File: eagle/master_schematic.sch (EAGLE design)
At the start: 110 parts

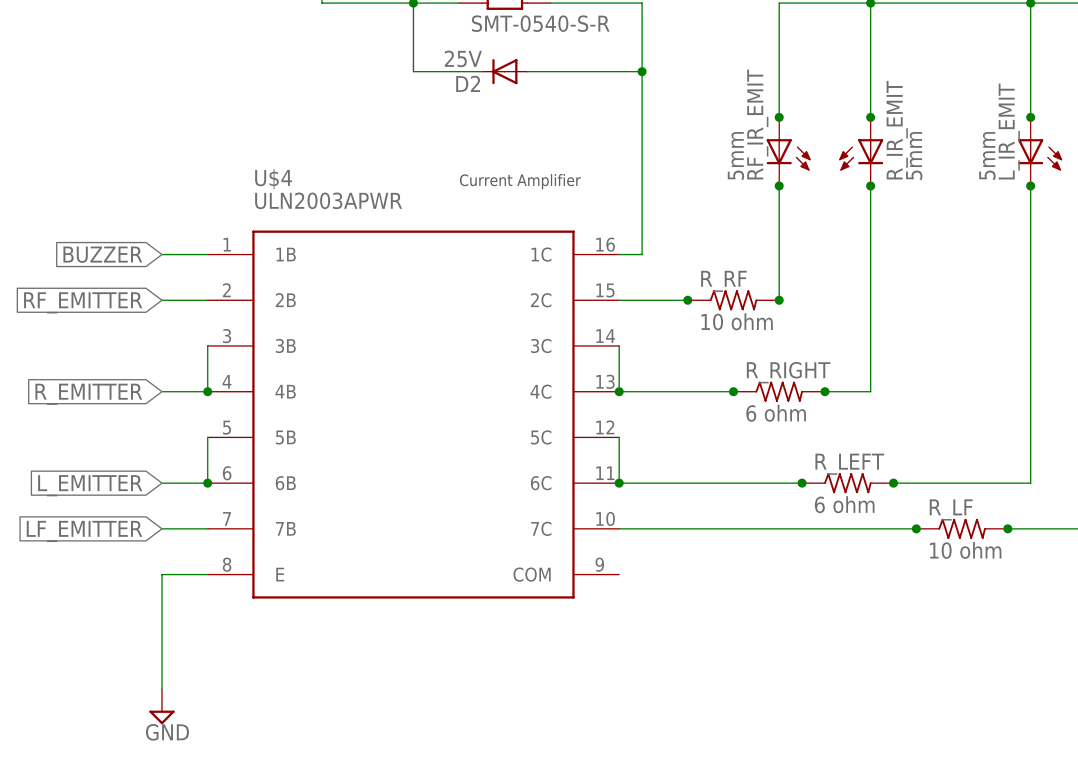
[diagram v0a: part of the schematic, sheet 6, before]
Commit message: ULN and stuff
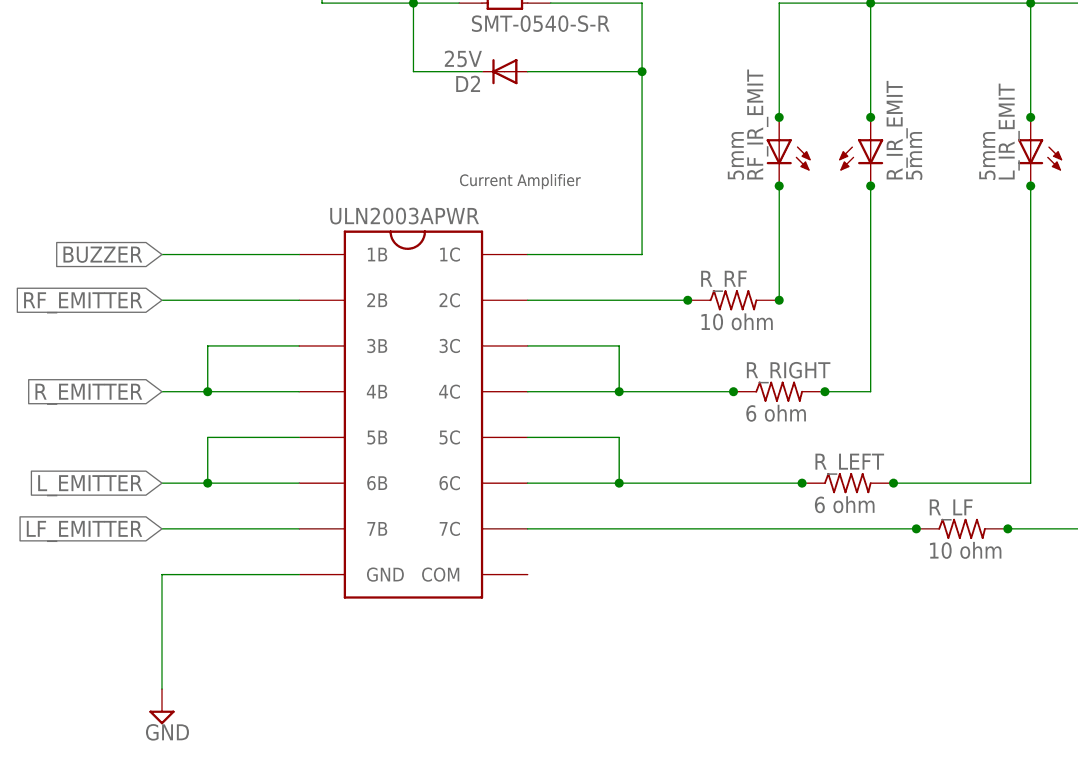
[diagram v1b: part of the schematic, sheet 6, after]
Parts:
- removed U$4: ULN2003APWR, MMULN:ULN2003APWR
- added U$9: ULN2003APWR, ULN2003APWR:ULN2003APWR
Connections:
- net BUZZER: now also U$9.1B; no longer U$4.1B
- net GND: now also U$9.GND; no longer U$4.E
- net LF_EMITTER: now also U$9.7B; no longer U$4.7B
- net L_EMITTER: now also U$9.5B, U$9.6B; no longer U$4.5B, U$4.6B
- net N$22: now also U$9.2C; no longer U$4.2C
- net N$24: now also U$9.3C, U$9.4C; no longer U$4.3C, U$4.4C
- net N$27: now also U$9.5C, U$9.6C; no longer U$4.5C, U$4.6C
- net N$29: now also U$9.1C; no longer U$4.1C
- net N$30: now also U$9.7C; no longer U$4.7C
- net RF_EMITTER: now also U$9.2B; no longer U$4.2B
- net R_EMITTER: now also U$9.3B, U$9.4B; no longer U$4.3B, U$4.4B
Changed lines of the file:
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@@
 <part name="C1_F_EMITS" library="resistor" deviceset="C-EU" device="C1206" value="4.7uF"/>
 <part name="C2_F_EMITS" library="resistor" deviceset="C-EU" device="C1206" value=".1uF"/>
-<part name="U$4" library="MMULN" deviceset="ULN2003APWR" device=""/>
 <part name="R_MOT" library="pinhead" deviceset="PINHD-2X3" device=""/>
 <part name="L_MOT" library="pinhead" deviceset="PINHD-2X3" device=""/>
@@
 <part name="U$7" library="JST_CONNECTOR_FEMALE. through hole" deviceset="JST_CONNECTOR_FEMALE" device=""/>
 <part name="U$8" library="JST_CONNECTOR_FEMALE. through hole" deviceset="JST_CONNECTOR_FEMALE" device=""/>
+<part name="U$9" library="ULN2003APWR" deviceset="ULN2003APWR" device=""/>
 </parts>
 <sheets>
@@
 <instance part="C1_F_EMITS" gate="G$1" x="147.32" y="27.94" rot="R180"/>
 <instance part="C2_F_EMITS" gate="G$1" x="165.1" y="27.94" rot="R180"/>
-<instance part="U$4" gate="G$1" x="-17.78" y="0"/>
 <instance part="SUPPLY10" gate="GND" x="81.28" y="-17.78"/>
 <instance part="SUPPLY11" gate="GND" x="-45.72" y="-33.02"/>
@@
 <instance part="SPK1" gate="G$1" x="-7.62" y="45.72"/>
 <instance part="D2" gate="G$1" x="-7.62" y="38.1" rot="R180"/>
+<instance part="U$9" gate="G$1" x="-17.78" y="-2.54"/>
 </instances>
 <busses>
@@
 <net name="RF_EMITTER" class="0">
 <segment>
-<wire x1="-45.72" y1="12.7" x2="-40.64" y2="12.7" width="0.1524" layer="91"/>
 <label x="-45.72" y="12.7" size="1.778" layer="95" rot="R180" xref="yes"/>
-<pinref part="U$4" gate="G$1" pin="2B"/>
+<pinref part="U$9" gate="G$1" pin="2B"/>
+<wire x1="-45.72" y1="12.7" x2="-30.48" y2="12.7" width="0.1524" layer="91"/>
 </segment>
 </net>
@@
 <wire x1="-40.64" y1="2.54" x2="-40.64" y2="7.62" width="0.1524" layer="91"/>
 <label x="-45.72" y="2.54" size="1.778" layer="95" rot="R180" xref="yes"/>
-<pinref part="U$4" gate="G$1" pin="3B"/>
-<pinref part="U$4" gate="G$1" pin="4B"/>
+<pinref part="U$9" gate="G$1" pin="3B"/>
+<wire x1="-40.64" y1="7.62" x2="-30.48" y2="7.62" width="0.1524" layer="91"/>
+<pinref part="U$9" gate="G$1" pin="4B"/>
+<wire x1="-40.64" y1="2.54" x2="-30.48" y2="2.54" width="0.1524" layer="91"/>
 <junction x="-40.64" y="2.54"/>
 </segment>
@@
 <wire x1="-40.64" y1="-7.62" x2="-40.64" y2="-2.54" width="0.1524" layer="91"/>
 <label x="-45.72" y="-7.62" size="1.778" layer="95" rot="R180" xref="yes"/>
-<pinref part="U$4" gate="G$1" pin="5B"/>
-<pinref part="U$4" gate="G$1" pin="6B"/>
+<pinref part="U$9" gate="G$1" pin="5B"/>
+<wire x1="-40.64" y1="-2.54" x2="-30.48" y2="-2.54" width="0.1524" layer="91"/>
+<pinref part="U$9" gate="G$1" pin="6B"/>
+<wire x1="-40.64" y1="-7.62" x2="-30.48" y2="-7.62" width="0.1524" layer="91"/>
 <junction x="-40.64" y="-7.62"/>
 </segment>
@@
 <net name="LF_EMITTER" class="0">
 <segment>
-<wire x1="-40.64" y1="-12.7" x2="-45.72" y2="-12.7" width="0.1524" layer="91"/>
 <label x="-45.72" y="-12.7" size="1.778" layer="95" rot="R180" xref="yes"/>
-<pinref part="U$4" gate="G$1" pin="7B"/>
+<pinref part="U$9" gate="G$1" pin="7B"/>
+<wire x1="-45.72" y1="-12.7" x2="-30.48" y2="-12.7" width="0.1524" layer="91"/>
 </segment>
 </net>
@@
 <pinref part="R_RF" gate="G$1" pin="1"/>
 <junction x="12.7" y="12.7"/>
-<wire x1="12.7" y1="12.7" x2="5.08" y2="12.7" width="0.1524" layer="91"/>
-<pinref part="U$4" gate="G$1" pin="2C"/>
+<pinref part="U$9" gate="G$1" pin="2C"/>
+<wire x1="12.7" y1="12.7" x2="-5.08" y2="12.7" width="0.1524" layer="91"/>
 </segment>
 </net>
@@
 <wire x1="5.08" y1="7.62" x2="5.08" y2="2.54" width="0.1524" layer="91"/>
 <wire x1="17.78" y1="2.54" x2="5.08" y2="2.54" width="0.1524" layer="91"/>
-<pinref part="U$4" gate="G$1" pin="4C"/>
+<pinref part="U$9" gate="G$1" pin="4C"/>
+<wire x1="5.08" y1="2.54" x2="-5.08" y2="2.54" width="0.1524" layer="91"/>
 <junction x="5.08" y="2.54"/>
-<pinref part="U$4" gate="G$1" pin="3C"/>
+<pinref part="U$9" gate="G$1" pin="3C"/>
+<wire x1="5.08" y1="7.62" x2="-5.08" y2="7.62" width="0.1524" layer="91"/>
 </segment>
 </net>
@@
 <wire x1="5.08" y1="-2.54" x2="5.08" y2="-7.62" width="0.1524" layer="91"/>
 <wire x1="25.4" y1="-7.62" x2="5.08" y2="-7.62" width="0.1524" layer="91"/>
-<pinref part="U$4" gate="G$1" pin="6C"/>
+<pinref part="U$9" gate="G$1" pin="5C"/>
+<wire x1="5.08" y1="-2.54" x2="-5.08" y2="-2.54" width="0.1524" layer="91"/>
+<pinref part="U$9" gate="G$1" pin="6C"/>
+<wire x1="5.08" y1="-7.62" x2="-5.08" y2="-7.62" width="0.1524" layer="91"/>
 <junction x="5.08" y="-7.62"/>
-<pinref part="U$4" gate="G$1" pin="5C"/>
 </segment>
 </net>
@@
 <pinref part="R_LF" gate="G$1" pin="1"/>
 <junction x="38.1" y="-12.7"/>
-<wire x1="38.1" y1="-12.7" x2="5.08" y2="-12.7" width="0.1524" layer="91"/>
-<pinref part="U$4" gate="G$1" pin="7C"/>
+<wire x1="38.1" y1="-12.7" x2="-5.08" y2="-12.7" width="0.1524" layer="91"/>
+<pinref part="U$9" gate="G$1" pin="7C"/>
 </segment>
 </net>
 <net name="GND" class="0">
 <segment>
-<wire x1="-40.64" y1="-17.78" x2="-45.72" y2="-17.78" width="0.1524" layer="91"/>
 <wire x1="-45.72" y1="-17.78" x2="-45.72" y2="-30.48" width="0.1524" layer="91"/>
-<pinref part="U$4" gate="G$1" pin="E"/>
 <pinref part="SUPPLY11" gate="GND" pin="GND"/>
+<pinref part="U$9" gate="G$1" pin="GND"/>
+<wire x1="-45.72" y1="-17.78" x2="-30.48" y2="-17.78" width="0.1524" layer="91"/>
 </segment>
 <segment>
@@
 <net name="BUZZER" class="0">
 <segment>
-<pinref part="U$4" gate="G$1" pin="1B"/>
-<wire x1="-40.64" y1="17.78" x2="-45.72" y2="17.78" width="0.1524" layer="91"/>
 <label x="-45.72" y="17.78" size="1.778" layer="95" rot="R180" xref="yes"/>
+<pinref part="U$9" gate="G$1" pin="1B"/>
+<wire x1="-45.72" y1="17.78" x2="-30.48" y2="17.78" width="0.1524" layer="91"/>
 </segment>
 </net>
 <net name="N$29" class="0">
 <segment>
-<pinref part="U$4" gate="G$1" pin="1C"/>
-<wire x1="7.62" y1="17.78" x2="5.08" y2="17.78" width="0.1524" layer="91"/>
 <pinref part="SPK1" gate="G$1" pin="-"/>
 <wire x1="-2.54" y1="45.72" x2="7.62" y2="45.72" width="0.1524" layer="91"/>
@@
 <wire x1="-5.08" y1="38.1" x2="7.62" y2="38.1" width="0.1524" layer="91"/>
 <junction x="7.62" y="38.1"/>
-</segment>
-</net>
+<pinref part="U$9" gate="G$1" pin="1C"/>
+<wire x1="7.62" y1="17.78" x2="-5.08" y2="17.78" width="0.1524" layer="91"/>
+</segment>
+</net>
